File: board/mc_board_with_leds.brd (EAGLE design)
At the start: 75.2 x 36.8 mm, 36 parts, among them IC1 TPS61070DDC, IC2 MEGA8-P, Q2 16MHz

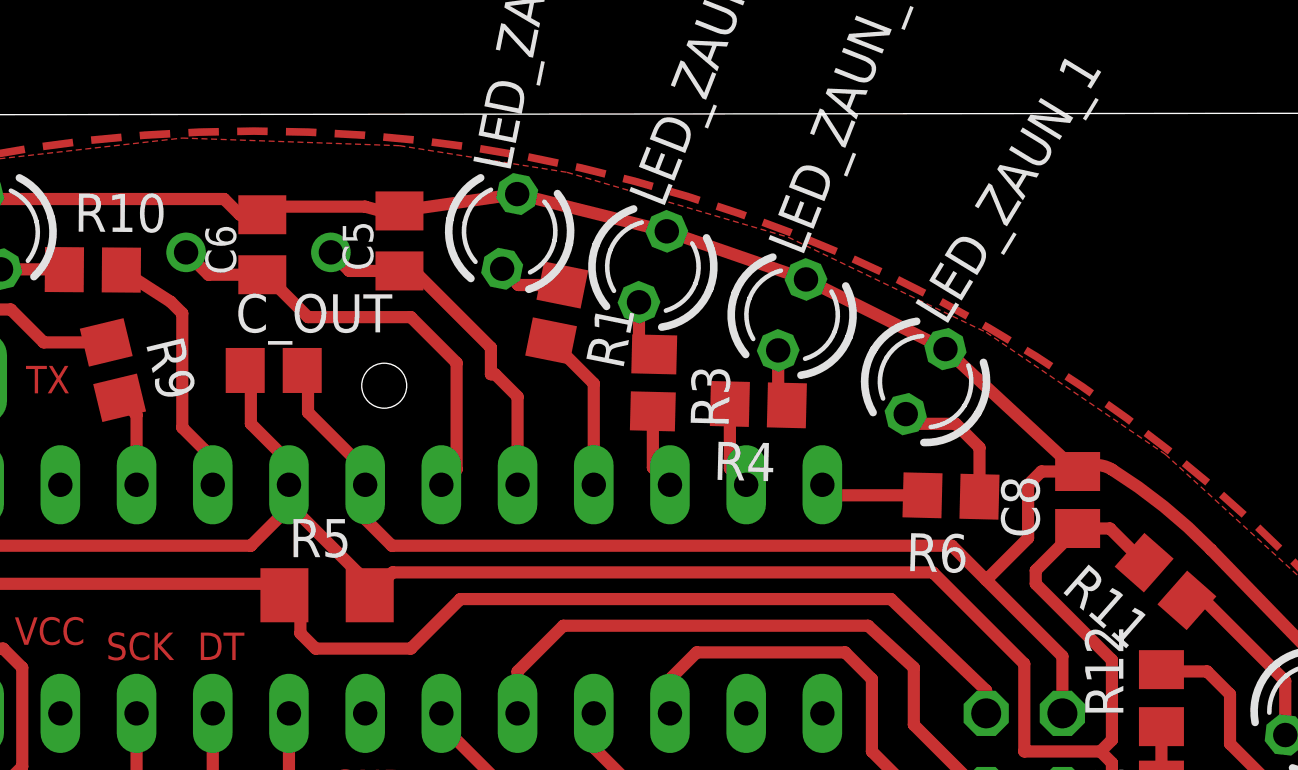
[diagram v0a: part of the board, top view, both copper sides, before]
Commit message: replaced some things on the board
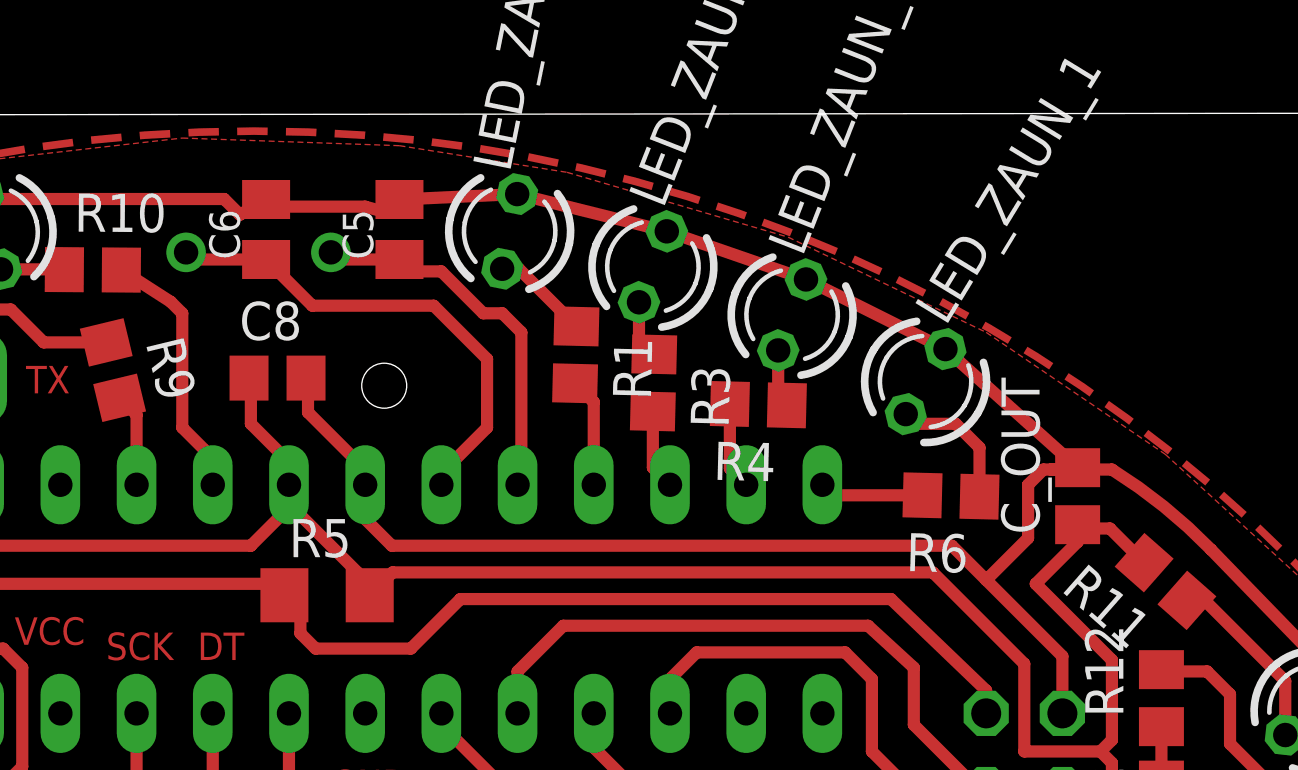
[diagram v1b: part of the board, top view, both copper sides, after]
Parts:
- moved C_OUT 27.1 mm to (76.5, 36.8), turned to 90 degrees
- moved C8 27.0 mm to (49.8, 40.8), turned to 0 degrees
- moved R1 1.53 mm to (59.7, 41.5), turned to 268.6 degrees
- moved C6 0.52 mm to (49.4, 45.7)
- moved C5 0.38 mm to (53.8, 45.7)
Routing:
- net PD5/LED_ZAUN_4: track 5.39 -> 3.64 mm
- net N$14: track 14.8 -> 16.3 mm
- net N$4: track 11.7 -> 12.8 mm
- net N$1: track 2.23 -> 3.27 mm
- net GND: track 193.5 -> 194.3 mm

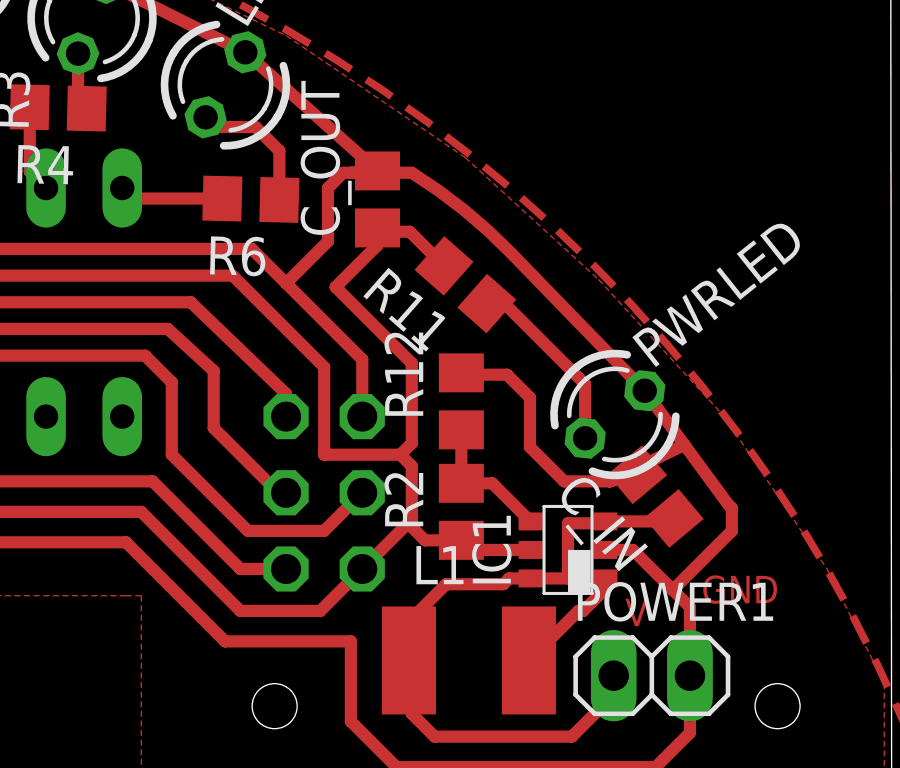
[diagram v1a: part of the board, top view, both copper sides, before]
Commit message: added missing values
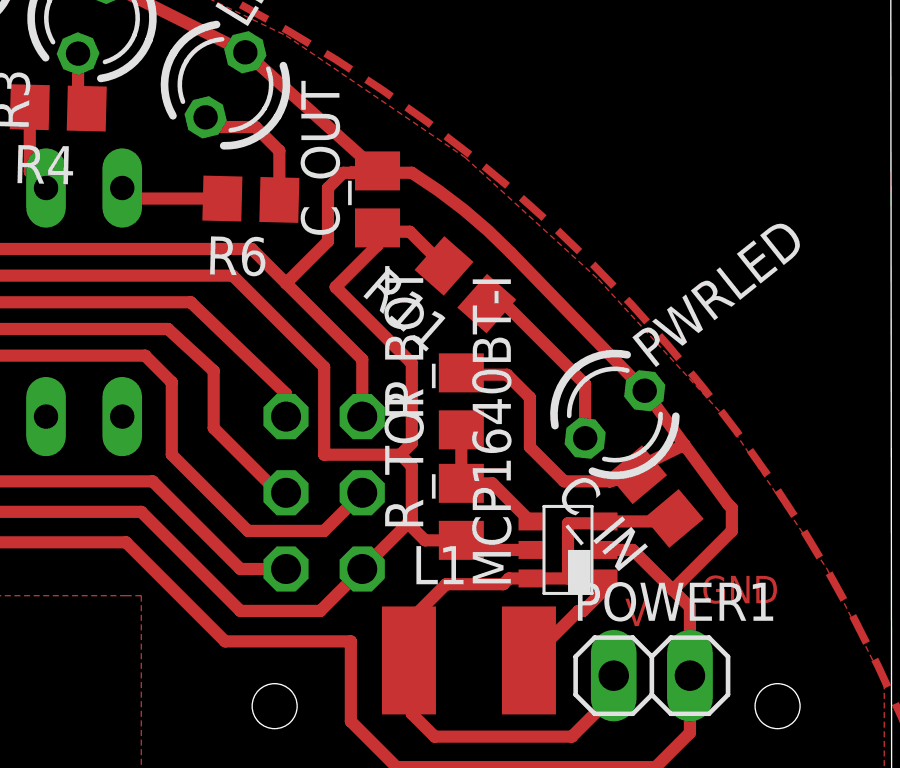
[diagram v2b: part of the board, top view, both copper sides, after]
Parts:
- C_IN: value (none) -> 4.7μF
- C_OUT: value (none) -> 47μF
- L1: value (none) -> 4,7µH
- R_BOT: value (none) -> 330k
- R_TOP: value (none) -> 560k
- renumbered IC1 to MCP1640BT-I, R12 to R_BOT, R2 to R_TOP
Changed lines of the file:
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@@
 <element name="HX1" library="pinhead" package="1X04" value="JP1" x="46.355" y="26.162" rot="MR0"/>
 <element name="UART1" library="pinhead" package="1X02" value="JP2" x="38.735" y="40.767" rot="MR180"/>
-<element name="IC1" library="texas" package="TSOT23-6_DDC" value="TPS61070DDC" x="82.804" y="25.146" rot="R90">
+<element name="MCP1640BT-I" library="texas" package="TSOT23-6_DDC" value="TPS61070DDC" x="82.804" y="25.146" rot="R90">
 <attribute name="MPN" value="TPS61070DDCR" x="82.804" y="25.146" size="1.778" layer="27" rot="R90" display="off"/>
 <attribute name="OC_NEWARK" value="64M3125" x="82.804" y="25.146" size="1.778" layer="27" rot="R90" display="off"/>
@@
 <attribute name="OC_FARNELL" value="1461062" x="82.804" y="25.146" size="1.778" layer="27" rot="R90" display="off"/>
 </element>
-<element name="L1" library="rcl" package="L4532P" value="" x="79.502" y="21.463"/>
-<element name="R2" library="resistor" package="R0805" value="" x="79.248" y="26.416" rot="R90"/>
-<element name="R12" library="resistor" package="R0805" value="" x="79.248" y="30.099" rot="R90"/>
-<element name="C_IN" library="rcl-2" package="C0805" value="" x="85.725" y="26.924" rot="R130"/>
-<element name="C_OUT" library="rcl-2" package="C0805" value="" x="76.454" y="36.83" rot="R90"/>
+<element name="L1" library="rcl" package="L4532P" value="4,7µH" x="79.502" y="21.463"/>
+<element name="R_TOP" library="resistor" package="R0805" value="560k" x="79.248" y="26.416" rot="R90"/>
+<element name="R_BOT" library="resistor" package="R0805" value="330k" x="79.248" y="30.099" rot="R90"/>
+<element name="C_IN" library="rcl-2" package="C0805" value="4.7μF" x="85.725" y="26.924" rot="R130"/>
+<element name="C_OUT" library="rcl-2" package="C0805" value="47μF" x="76.454" y="36.83" rot="R90"/>
 </elements>
 <signals>
@@
 <wire x1="25.273" y1="32.893" x2="25.273" y2="34.798" width="0.4064" layer="1"/>
 <wire x1="25.273" y1="34.798" x2="23.368" y2="36.703" width="0.4064" layer="1"/>
-<contactref element="IC1" pad="2"/>
+<contactref element="MCP1640BT-I" pad="2"/>
 <contactref element="C_IN" pad="2"/>
 <contactref element="C_OUT" pad="2"/>
-<contactref element="R12" pad="2"/>
+<contactref element="R_BOT" pad="2"/>
 <wire x1="28.5496" y1="29.6164" x2="25.273" y2="32.893" width="0.4064" layer="1"/>
 <wire x1="49.403" y1="46.72" x2="49.927" y2="46.482" width="0.4064" layer="1"/>
@@
 <wire x1="35.433" y1="39.497" x2="34.036" y2="39.497" width="0.4064" layer="1"/>
 <wire x1="34.036" y1="39.497" x2="33.081" y2="38.542" width="0.4064" layer="1"/>
-<contactref element="IC1" pad="5"/>
-<contactref element="R2" pad="1"/>
+<contactref element="MCP1640BT-I" pad="5"/>
+<contactref element="R_TOP" pad="1"/>
 <contactref element="C_OUT" pad="1"/>
 <wire x1="33.081" y1="38.542" x2="33.081" y2="35.88" width="0.4064" layer="1"/>
@@
 <signal name="V_IN">
 <contactref element="POWER1" pad="1"/>
-<contactref element="IC1" pad="6"/>
+<contactref element="MCP1640BT-I" pad="6"/>
 <contactref element="C_IN" pad="1"/>
 <contactref element="L1" pad="1"/>
-<contactref element="IC1" pad="3"/>
+<contactref element="MCP1640BT-I" pad="3"/>
 <wire x1="81.554" y1="24.196" x2="82.804" y2="24.196" width="0.4064" layer="1"/>
 <wire x1="82.804" y1="24.196" x2="82.804" y2="26.035" width="0.4064" layer="1"/>
@@
 </signal>
 <signal name="N$5">
-<contactref element="IC1" pad="1"/>
+<contactref element="MCP1640BT-I" pad="1"/>
 <contactref element="L1" pad="2"/>
 <wire x1="84.074" y1="24.176" x2="84.054" y2="24.196" width="0.4064" layer="1"/>
@@
 </signal>
 <signal name="N$6">
-<contactref element="R12" pad="1"/>
-<contactref element="R2" pad="2"/>
-<contactref element="IC1" pad="4"/>
+<contactref element="R_BOT" pad="1"/>
+<contactref element="R_TOP" pad="2"/>
+<contactref element="MCP1640BT-I" pad="4"/>
 <wire x1="79.248" y1="27.366" x2="79.248" y2="29.149" width="0.4064" layer="1"/>
 <wire x1="81.554" y1="26.096" x2="80.284" y2="27.366" width="0.4064" layer="1"/>
